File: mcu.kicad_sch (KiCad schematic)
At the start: 47 parts, among them J1 USB_B, J2 Conn_01x05_Pin, SW1 SW_Push, U1 STM32F103CBTx, U2 USB6B1, U3 AMS1117-3.3, Y1 8Mhz

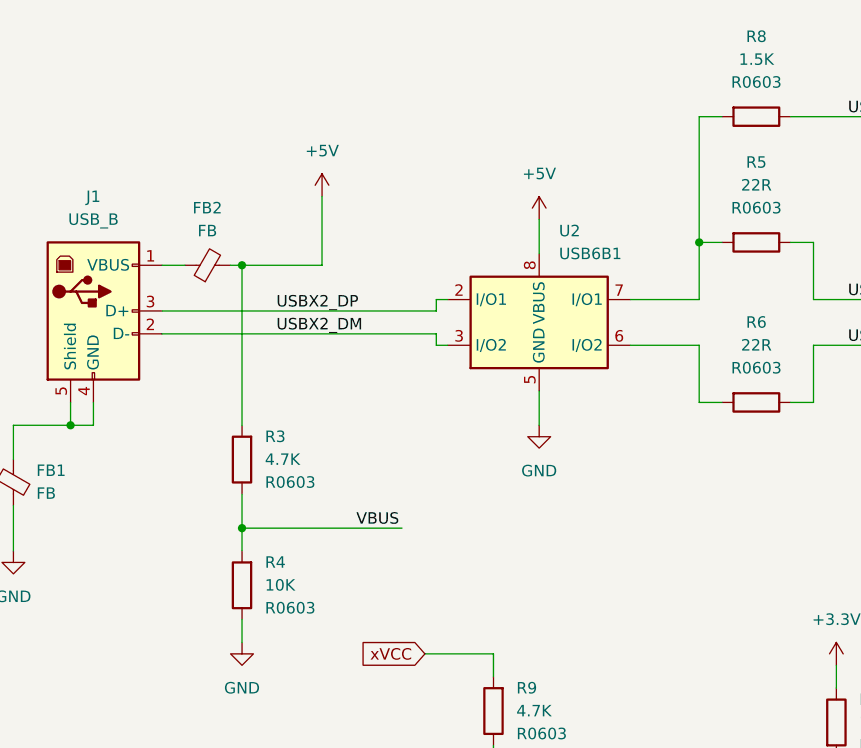
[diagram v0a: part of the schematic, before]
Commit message: update
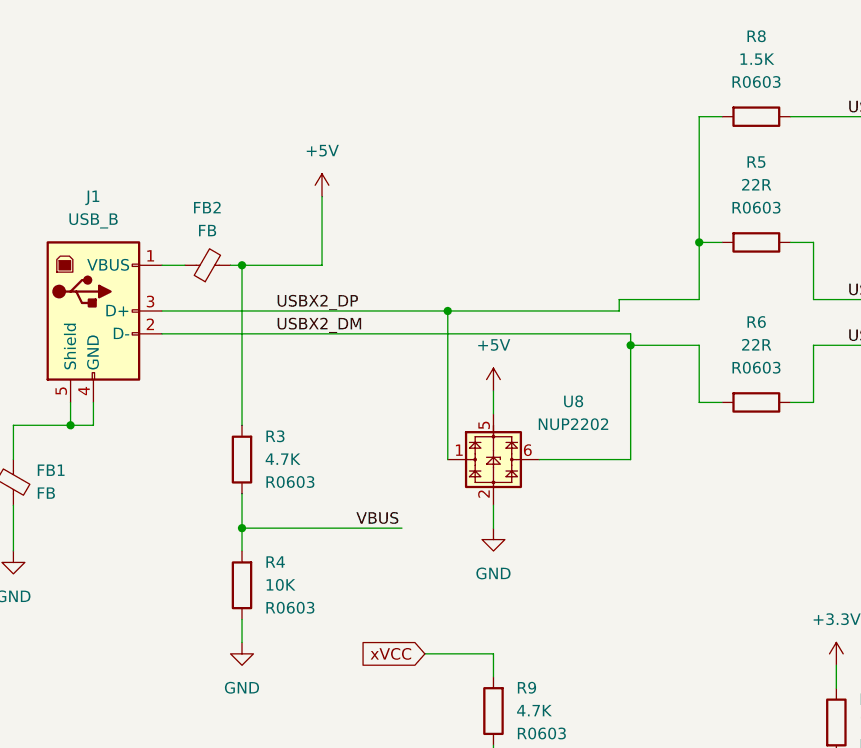
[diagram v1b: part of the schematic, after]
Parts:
- removed U2: USB6B1, Package_SO:SOIC-8_3.9x4.9mm_P1.27mm, symbol Power_Protection:USB6B1
- added U8: NUP2202, Package_TO_SOT_SMD:SOT-363_SC-70-6, symbol Power_Protection:NUP2202
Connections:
- net +5V: now also U8.5
- net GND: now also U8.2
- net USBX2_DM: now also R6.2, U8.6
- net USBX2_DP: now also R5.2, R8.2, U8.1
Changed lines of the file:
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@@
 	)
 	(junction
+		(at 86.36 92.71)
+		(diameter 0)
+		(color 0 0 0 0)
+	)
+	(junction
 		(at 176.53 71.12)
 		(diameter 0)
@@
 	)
 	(junction
+		(at 66.04 88.9)
+		(diameter 0)
+		(color 0 0 0 0)
+	)
+	(junction
 		(at 113.03 31.75)
 		(diameter 0)
@@
 	(wire
 		(pts
+			(xy 86.36 91.44) (xy 86.36 92.71)
+		)
+		(stroke
+			(width 0)
+			(type default)
+		)
+	)
+	(wire
+		(pts
 			(xy 190.5 55.88) (xy 190.5 68.58)
 		)
@@
 	(wire
 		(pts
-			(xy 86.36 87.63) (xy 93.98 87.63)
-		)
-		(stroke
-			(width 0)
-			(type default)
-		)
-	)
-	(wire
-		(pts
 			(xy 198.12 114.3) (xy 212.09 114.3)
 		)
@@
 	(wire
 		(pts
-			(xy 64.77 88.9) (xy 64.77 87.63)
-		)
-		(stroke
-			(width 0)
-			(type default)
-		)
-	)
-	(wire
-		(pts
 			(xy 104.14 81.28) (xy 106.68 81.28)
 		)
@@
 	(wire
 		(pts
-			(xy 64.77 91.44) (xy 64.77 92.71)
+			(xy 71.12 110.49) (xy 71.12 113.03)
 		)
 		(stroke
@@
 	(wire
 		(pts
-			(xy 64.77 87.63) (xy 66.04 87.63)
-		)
-		(stroke
-			(width 0)
-			(type default)
-		)
-	)
-	(wire
-		(pts
 			(xy 128.27 186.69) (xy 128.27 189.23)
 		)
@@
 	(wire
 		(pts
-			(xy 76.2 97.79) (xy 76.2 101.6)
-		)
-		(stroke
-			(width 0)
-			(type default)
-		)
-	)
-	(wire
-		(pts
 			(xy 24.13 99.06) (xy 24.13 101.6)
 		)
@@
 	(wire
 		(pts
+			(xy 76.2 105.41) (xy 86.36 105.41)
+		)
+		(stroke
+			(width 0)
+			(type default)
+		)
+	)
+	(wire
+		(pts
 			(xy 173.99 146.05) (xy 173.99 149.86)
 		)
@@
 	(wire
 		(pts
-			(xy 64.77 92.71) (xy 66.04 92.71)
+			(xy 66.04 88.9) (xy 66.04 105.41)
+		)
+		(stroke
+			(width 0)
+			(type default)
+		)
+	)
+	(wire
+		(pts
+			(xy 85.09 87.63) (xy 93.98 87.63)
 		)
 		(stroke
@@
 	(wire
 		(pts
-			(xy 34.29 91.44) (xy 64.77 91.44)
+			(xy 34.29 91.44) (xy 86.36 91.44)
+		)
+		(stroke
+			(width 0)
+			(type default)
+		)
+	)
+	(wire
+		(pts
+			(xy 85.09 88.9) (xy 85.09 87.63)
 		)
 		(stroke
@@
 	(wire
 		(pts
+			(xy 71.12 97.79) (xy 71.12 100.33)
+		)
+		(stroke
+			(width 0)
+			(type default)
+		)
+	)
+	(wire
+		(pts
 			(xy 229.87 25.4) (xy 229.87 21.59)
 		)
@@
 	(wire
 		(pts
-			(xy 76.2 78.74) (xy 76.2 82.55)
-		)
-		(stroke
-			(width 0)
-			(type default)
-		)
-	)
-	(wire
-		(pts
 			(xy 228.6 135.89) (xy 229.87 135.89)
 		)
@@
 	(wire
 		(pts
-			(xy 34.29 88.9) (xy 64.77 88.9)
+			(xy 34.29 88.9) (xy 66.04 88.9)
 		)
 		(stroke
@@
 	(wire
 		(pts
+			(xy 86.36 105.41) (xy 86.36 92.71)
+		)
+		(stroke
+			(width 0)
+			(type default)
+		)
+	)
+	(wire
+		(pts
 			(xy 24.13 31.75) (xy 24.13 34.29)
 		)
@@
 	(wire
 		(pts
+			(xy 66.04 88.9) (xy 85.09 88.9)
+		)
+		(stroke
+			(width 0)
+			(type default)
+		)
+	)
+	(wire
+		(pts
 			(xy 106.68 87.63) (xy 120.65 87.63)
 		)
@@
 	)
 	(symbol
+		(lib_id "Power_Protection:NUP2202")
+		(at 71.12 105.41 0)
+		(unit 1)
+		(exclude_from_sim no)
+		(in_bom yes)
+		(on_board yes)
+		(dnp no)
+		(fields_autoplaced yes)
+		(property "Reference" "U8"
+			(at 80.01 98.9898 0)
+			(effects
+				(font
+					(size 1.27 1.27)
+				)
+			)
+		)
+		(property "Value" "NUP2202"
+			(at 80.01 101.5298 0)
+			(effects
+				(font
+					(size 1.27 1.27)
+				)
+			)
+		)
+		(property "Footprint" "Package_TO_SOT_SMD:SOT-363_SC-70-6"
+			(at 73.152 103.505 0)
+			(effects
+				(font
+					(size 1.27 1.27)
+				)
+				(hide yes)
+			)
+		)
+		(property "Datasheet" "https://www.onsemi.com/pdf/datasheet/nup2202w1-d.pdf"
+			(at 73.152 103.505 0)
+			(effects
+				(font
+					(size 1.27 1.27)
+				)
+				(hide yes)
+			)
+		)
+		(property "Description" "Transient voltage suppressor designed to protect high speed data lines from ESD, EFT, and lightning"
+			(at 71.12 105.41 0)
+			(effects
+				(font
+					(size 1.27 1.27)
+				)
+				(hide yes)
+			)
+		)
+		(pin "6"
+		)
+		(pin "2"
+		)
+		(pin "3"
+		)
+		(pin "5"
+		)
+		(pin "4"
+		)
+		(pin "1"
+		)
+		(instances
+			(project ""
+				(path "/c46f0577-8378-47ed-a184-c512ebaa7448/cf4a56a0-87cc-48b2-b91a-72f3bf53d7c4"
+					(reference "U8")
+					(unit 1)
+				)
+			)
+		)
+	)
+	(symbol
 		(lib_id "Device:C")
 		(at 229.87 29.21 0)
@@
 	)
 	(symbol
-		(lib_id "Power_Protection:USB6B1")
-		(at 76.2 90.17 0)
-		(unit 1)
-		(exclude_from_sim no)
-		(in_bom yes)
-		(on_board yes)
-		(dnp no)
-		(fields_autoplaced yes)
-		(property "Reference" "U2"
-			(at 78.3941 80.01 0)
-			(effects
-				(font
-					(size 1.27 1.27)
-				)
-				(justify left)
-			)
-		)
-		(property "Value" "USB6B1"
-			(at 78.3941 82.55 0)
-			(effects
-				(font
-					(size 1.27 1.27)
-				)
-				(justify left)
-			)
-		)
-		(property "Footprint" "Package_SO:SOIC-8_3.9x4.9mm_P1.27mm"
-			(at 76.2 90.17 0)
-			(effects
-				(font
-					(size 1.27 1.27)
-				)
-				(hide yes)
-			)
-		)
-		(property "Datasheet" "http://www.st.com/content/ccc/resource/technical/document/datasheet/3e/ec/b2/54/b2/76/47/90/CD00001361.pdf/files/CD00001361.pdf/jcr:content/translations/en.CD00001361.pdf"
-			(at 52.07 92.71 0)
-			(effects
-				(font
-					(size 1.27 1.27)
-				)
-				(hide yes)
-			)
-		)
-		(property "Description" "5V Data line protection"
-			(at 76.2 90.17 0)
-			(effects
-				(font
-					(size 1.27 1.27)
-				)
-				(hide yes)
-			)
-		)
-		(pin "8"
-		)
-		(pin "1"
-		)
-		(pin "2"
-		)
-		(pin "6"
-		)
-		(pin "4"
-		)
-		(pin "7"
-		)
-		(pin "3"
-		)
-		(pin "5"
-		)
-		(instances
-			(project ""
-				(path "/c46f0577-8378-47ed-a184-c512ebaa7448/cf4a56a0-87cc-48b2-b91a-72f3bf53d7c4"
-					(reference "U2")
-					(unit 1)
-				)
-			)
-		)
-	)
-	(symbol
 		(lib_id "power:GND")
 		(at 17.78 115.57 0)
@@
 	(symbol
 		(lib_id "power:+5V")
-		(at 76.2 78.74 0)
+		(at 71.12 97.79 0)
 		(unit 1)
 		(exclude_from_sim no)
@@
 		(fields_autoplaced yes)
 		(property "Reference" "#PWR04"
-			(at 76.2 82.55 0)
+			(at 71.12 101.6 0)
 			(effects
 				(font
@@
 		)
 		(property "Value" "+5V"
-			(at 76.2 73.66 0)
+			(at 71.12 92.71 0)
 			(effects
 				(font
@@
 		)
 		(property "Footprint" ""
-			(at 76.2 78.74 0)
+			(at 71.12 97.79 0)
 			(effects
 				(font
@@
 		)
 		(property "Datasheet" ""
-			(at 76.2 78.74 0)
+			(at 71.12 97.79 0)
 			(effects
 				(font
@@
 		)
 		(property "Description" "Power symbol creates a global label with name \"+5V\""
-			(at 76.2 78.74 0)
+			(at 71.12 97.79 0)
 			(effects
 				(font
@@
 	(symbol
 		(lib_id "power:GND")
-		(at 76.2 101.6 0)
+		(at 71.12 113.03 0)
 		(unit 1)
 		(exclude_from_sim no)
@@
 		(fields_autoplaced yes)
 		(property "Reference" "#PWR05"
-			(at 76.2 107.95 0)
+			(at 71.12 119.38 0)
 			(effects
 				(font
@@
 		)
 		(property "Value" "GND"
-			(at 76.2 106.68 0)
+			(at 71.12 118.11 0)
 			(effects
 				(font
@@
 		)
 		(property "Footprint" ""
-			(at 76.2 101.6 0)
+			(at 71.12 113.03 0)
 			(effects
 				(font
@@
 		)
 		(property "Datasheet" ""
-			(at 76.2 101.6 0)
+			(at 71.12 113.03 0)
 			(effects
 				(font
@@
 		)
 		(property "Description" "Power symbol creates a global label with name \"GND\" , ground"
-			(at 76.2 101.6 0)
+			(at 71.12 113.03 0)
 			(effects
 				(font
